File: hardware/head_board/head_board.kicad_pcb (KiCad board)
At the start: 2 copper layers, 90 x 74.7 mm, 121 parts, among them J1 8P8C, J2 CAM, J3 MOTOR, J4 MOTOR, J5 MOTOR, J6 CAMLED, SW1 BOOTSEL, U1 P78E05-1000, U2 MIC5317-3.3, U3 RP2040, U4 TVS, U5 W25Q128JVS, U6 TMC2209, U7 TMC2209, U8 TMC2209, U9 74HC2G34, Y1 12MHz

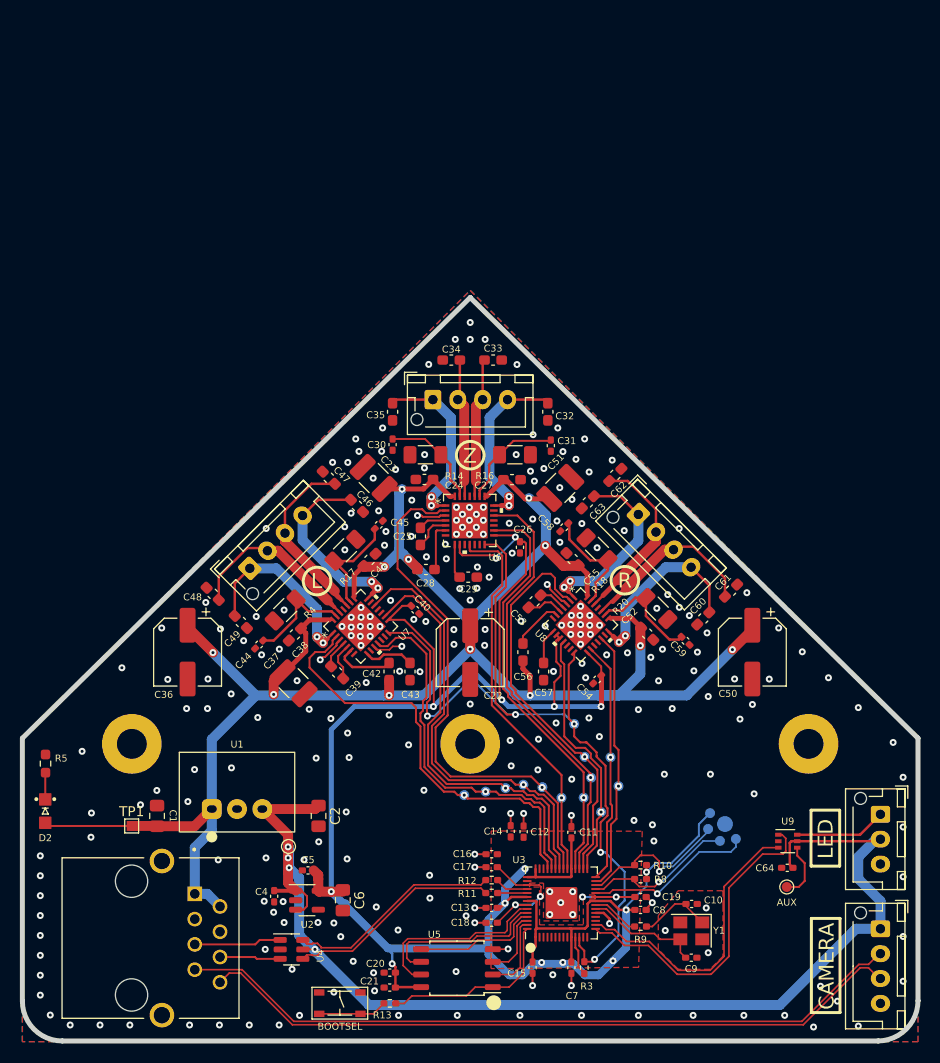
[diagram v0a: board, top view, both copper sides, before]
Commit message: Finish up layout for v1, ended up removing some stuff
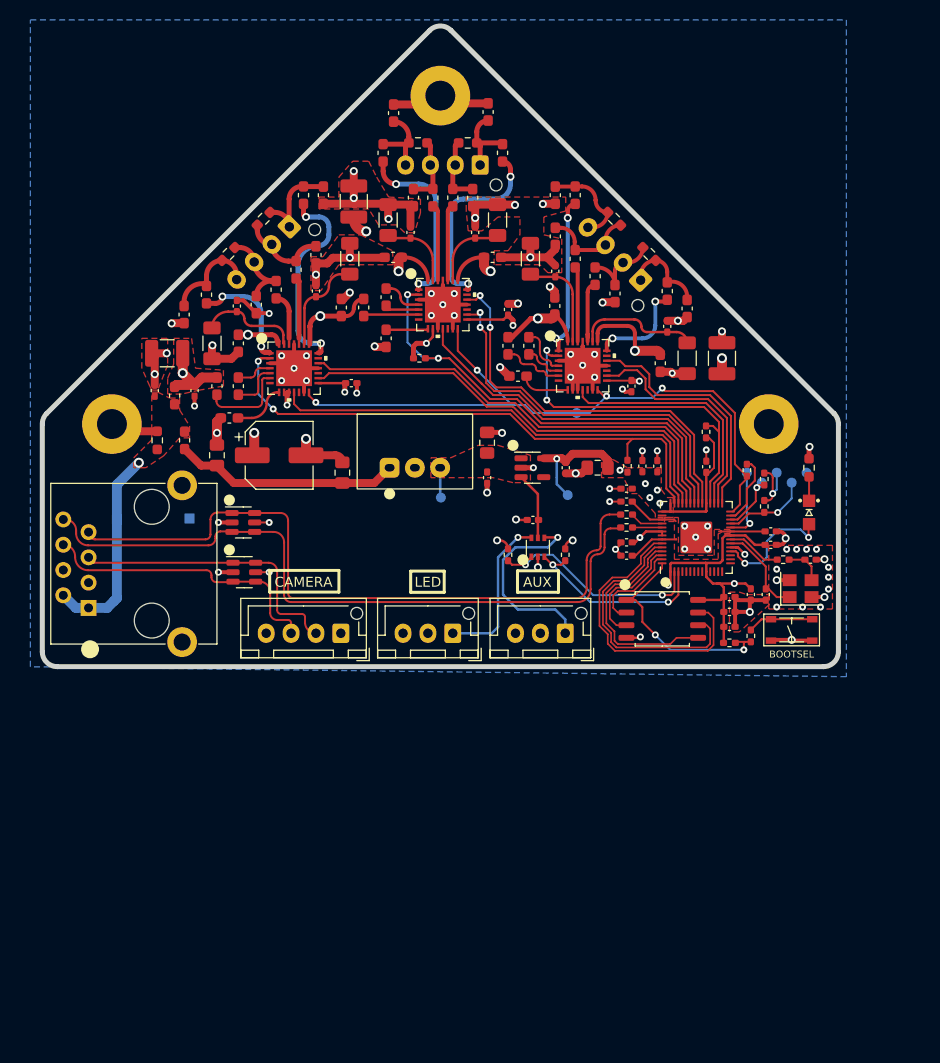
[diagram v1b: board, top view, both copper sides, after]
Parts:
- removed C1: 22u, Capacitor_SMD:C_0805_2012Metric_Pad1.18x1.45mm_HandSolder
- removed C22: 100u, Capacitor_SMD:CP_Elec_6.3x7.7
- removed the C25 at (103.2, 91.9)
- removed the C26 at (113.2, 93.0)
- removed the C28 at (103.8, 95.2)
- removed the C29 at (108.0, 96.0)
- removed the C36 at (79.8, 103.5)
- removed the C50 at (136.6, 103.5)
- removed the C64 at (140.1, 125.2)
- removed D2: 24V, winterbloom:LED_0805_Kingbright_APT2012
- removed G***: LOGO, winterbloom:Symbol_Winterbloom_40mm
- removed J1: 8P8C, winterbloom:Connector_RJ45_SS-7188S-A-PG4-BA-50
- removed J6: CAMLED, Connector_JST:JST_XH_B3B-XH-AM_1x03_P2.50mm_Vertical
- removed the R5 at (65.5, 114.7)
- removed TP10: M2STP, TestPoint:TestPoint_Pad_D1.0mm
- removed TP11: M2DAG, TestPoint:TestPoint_Pad_D1.0mm
- removed TP12: M2EN, TestPoint:TestPoint_Pad_D1.0mm
- removed TP13: M1DIR, TestPoint:TestPoint_Pad_D1.0mm
- removed TP14: M1STP, TestPoint:TestPoint_Pad_D1.0mm
- removed TP15: M1DAG, TestPoint:TestPoint_Pad_D1.0mm
- removed TP16: M1EN, TestPoint:TestPoint_Pad_D1.0mm
- removed TP18: M0STP, TestPoint:TestPoint_Pad_D1.0mm
- removed TP19: M0DAG, TestPoint:TestPoint_Pad_D1.0mm
- removed TP20: M0EN, TestPoint:TestPoint_Pad_D1.0mm
- removed TP21: UART, TestPoint:TestPoint_Pad_D1.0mm
- removed TP22: AUX, TestPoint:TestPoint_Pad_D1.0mm
- removed the U4 at (90.2, 133.4)
- removed the U9 at (140.1, 122.5)
- added C10: 10u, Capacitor_SMD:C_0805_2012Metric_Pad1.18x1.45mm_HandSolder, F.Cu at (121.0, 85.0)
- added C27: 100n, Capacitor_SMD:C_0402_1005Metric_Pad0.74x0.62mm_HandSolder, F.Cu at (114.5, 90.2)
- added C3: 22u, Capacitor_SMD:C_0805_2012Metric_Pad1.18x1.45mm_HandSolder, F.Cu at (82.8, 83.8)
- added C42: 22n, Capacitor_SMD:C_0603_1608Metric_Pad1.08x0.95mm_HandSolder, F.Cu at (99.8, 67.9)
- added C43: 100n, Capacitor_SMD:C_0402_1005Metric_Pad0.74x0.62mm_HandSolder, F.Cu at (112.0, 69.1)
- added C44: 100n, Capacitor_SMD:C_0603_1608Metric_Pad1.08x0.95mm_HandSolder, F.Cu at (97.5, 68.9)
- added C45: 4.7u, Capacitor_SMD:C_0603_1608Metric_Pad1.08x0.95mm_HandSolder, F.Cu at (99.8, 72.0)
- added C7: 1u, Capacitor_SMD:C_0402_1005Metric_Pad0.74x0.62mm_HandSolder, F.Cu at (117.8, 85.0)
- added C8: 100n, Capacitor_SMD:C_0402_1005Metric_Pad0.74x0.62mm_HandSolder, F.Cu at (76.5, 77.2)
- added C9: 100n, Capacitor_SMD:C_0402_1005Metric_Pad0.74x0.62mm_HandSolder, F.Cu at (80.5, 77.2)
- added D4: ACT, winterbloom:LED_0805_Kingbright_APT2012, F.Cu at (142.2, 89.5)
- added FB1: 50Ω @ 100MHz, Inductor_SMD:L_0603_1608Metric_Pad1.05x0.95mm_HandSolder, F.Cu at (78.5, 77.8)
- added FB10: 50Ω @ 100MHz, Inductor_SMD:L_0603_1608Metric_Pad1.05x0.95mm_HandSolder, F.Cu at (81.7, 67.6)
- added FB11: 50Ω @ 100MHz, Inductor_SMD:L_0603_1608Metric_Pad1.05x0.95mm_HandSolder, F.Cu at (88.7, 67.1)
- added FB12: 50Ω @ 100MHz, Inductor_SMD:L_0603_1608Metric_Pad1.05x0.95mm_HandSolder, F.Cu at (90.7, 65.1)
- added FB13: 50Ω @ 100MHz, Inductor_SMD:L_0603_1608Metric_Pad1.05x0.95mm_HandSolder, F.Cu at (91.5, 57.6)
- added FB14: 50Ω @ 100MHz, Inductor_SMD:L_0603_1608Metric_Pad1.05x0.95mm_HandSolder, F.Cu at (79.5, 82.2)
- added FB2: 50Ω @ 100MHz, Inductor_SMD:L_0603_1608Metric_Pad1.05x0.95mm_HandSolder, F.Cu at (118.8, 57.6)
- added FB3: 50Ω @ 100MHz, Inductor_SMD:L_0603_1608Metric_Pad1.05x0.95mm_HandSolder, F.Cu at (118.8, 64.0)
- added FB4: 50Ω @ 100MHz, Inductor_SMD:L_0603_1608Metric_Pad1.05x0.95mm_HandSolder, F.Cu at (120.8, 65.8)
- added FB5: 50Ω @ 100MHz, Inductor_SMD:L_0603_1608Metric_Pad1.05x0.95mm_HandSolder, F.Cu at (128.0, 67.2)
- added FB6: 50Ω @ 100MHz, Inductor_SMD:L_0603_1608Metric_Pad1.05x0.95mm_HandSolder, F.Cu at (99.5, 53.4)
- added FB7: 50Ω @ 100MHz, Inductor_SMD:L_0603_1608Metric_Pad1.05x0.95mm_HandSolder, F.Cu at (104.5, 57.9)
- added FB8: 50Ω @ 100MHz, Inductor_SMD:L_0603_1608Metric_Pad1.05x0.95mm_HandSolder, F.Cu at (106.5, 57.9)
- added FB9: 50Ω @ 100MHz, Inductor_SMD:L_0603_1608Metric_Pad1.05x0.95mm_HandSolder, F.Cu at (111.5, 53.4)
- added J3: CAM, Connector_JST:JST_XH_B4B-XH-AM_1x04_P2.50mm_Vertical, F.Cu at (95.2, 101.6)
- added J4: CAMLED, Connector_JST:JST_XH_B3B-XH-AM_1x03_P2.50mm_Vertical, F.Cu at (106.5, 101.6)
- added J5: AUX, Connector_JST:JST_XH_B3B-XH-AM_1x03_P2.50mm_Vertical, F.Cu at (117.8, 101.6)
- added R10: 1k, Resistor_SMD:R_0603_1608Metric_Pad0.98x0.95mm_HandSolder, F.Cu at (142.2, 85.0)
- added R12: 10k, Resistor_SMD:R_0402_1005Metric_Pad0.72x0.64mm_HandSolder, F.Cu at (134.2, 102.6)
- added R13: 10k, Resistor_SMD:R_0402_1005Metric_Pad0.72x0.64mm_HandSolder, F.Cu at (112.0, 93.8)
- added R14: 10k, Resistor_SMD:R_0402_1005Metric_Pad0.72x0.64mm_HandSolder, F.Cu at (117.8, 93.8)
- added R17: 10k, Resistor_SMD:R_0402_1005Metric_Pad0.72x0.64mm_HandSolder, F.Cu at (131.9, 81.4)
- added R20: 10k, Resistor_SMD:R_0402_1005Metric_Pad0.72x0.64mm_HandSolder, F.Cu at (103.1, 74.0)
- added R23: 10k, Resistor_SMD:R_0402_1005Metric_Pad0.72x0.64mm_HandSolder, F.Cu at (124.0, 84.8)
- added RV1: 35V, Resistor_SMD:R_0603_1608Metric_Pad0.98x0.95mm_HandSolder, F.Cu at (76.8, 82.2)
- added RV2: 35V, Resistor_SMD:R_0603_1608Metric_Pad0.98x0.95mm_HandSolder, F.Cu at (122.7, 60.0)
- added RV3: 35V, Resistor_SMD:R_0603_1608Metric_Pad0.98x0.95mm_HandSolder, F.Cu at (126.2, 63.5)
- added RV4: 35V, Resistor_SMD:R_0603_1608Metric_Pad0.98x0.95mm_HandSolder, F.Cu at (103.0, 52.4)
- added RV5: 35V, Resistor_SMD:R_0603_1608Metric_Pad0.98x0.95mm_HandSolder, F.Cu at (108.0, 52.4)
- added RV6: 35V, Resistor_SMD:R_0603_1608Metric_Pad0.98x0.95mm_HandSolder, F.Cu at (83.9, 63.5)
- added RV7: 35V, Resistor_SMD:R_0603_1608Metric_Pad0.98x0.95mm_HandSolder, F.Cu at (87.4, 60.0)
- added U5: TVS, Package_TO_SOT_SMD:SOT-23-6, F.Cu at (85.5, 95.5)
- added U6: TVS, Package_TO_SOT_SMD:SOT-23-6, F.Cu at (85.4, 90.5)
- added U7: 74HC2G34, Package_TO_SOT_SMD:SOT-363_SC-70-6, F.Cu at (115.0, 93.0)
- C2: value 22u -> 4.7u
- C4: value 1u -> 22u; footprint Capacitor_SMD:C_0402_1005Metric_Pad0.74x0.62mm_HandSolder -> Capacitor_SMD:C_0805_2012Metric_Pad1.18x1.45mm_HandSolder
- C5: value 1u -> 100u; footprint Capacitor_SMD:C_0402_1005Metric_Pad0.74x0.62mm_HandSolder -> Capacitor_SMD:CP_Elec_6.3x7.7
- C6: value 10u -> 1u; footprint Capacitor_SMD:C_0805_2012Metric_Pad1.18x1.45mm_HandSolder -> Capacitor_SMD:C_0402_1005Metric_Pad0.74x0.62mm_HandSolder
- J2: value CAM -> 8P8C; footprint Connector_JST:JST_XH_B4B-XH-AM_1x04_P2.50mm_Vertical -> winterbloom:Connector_RJ45_ASSMANN_A-2014-2S-4-N-R
- J7: renamed from J4; moved to B.Cu
- J8: renamed from J3; moved to B.Cu
- J9: renamed from J5; moved to B.Cu
- R11: renamed from R9; value 1K -> 1k
- R18: renamed from R4; value 22R -> 220m
- R19: renamed from R17; value 22R -> 220m
- R21: renamed from R14; value 22R -> 220m
- R22: renamed from R16; value 22R -> 220m
- R24: renamed from R18; value 22R -> 220m
- R25: renamed from R20; value 22R -> 220m
- R4: renamed from R10; value 10K -> 10k
- R5: renamed from R8; value 10K -> 10k
- R8: renamed from R3; value 1K -> 1k
- R9: renamed from R13; value 1K -> 1k
- TP1: value 24V -> GND; moved to B.Cu
- TP17: value M0DIR -> UART
- TP2: value 5V -> 24V; footprint TestPoint:TestPoint_Pad_D1.0mm -> TestPoint:TestPoint_Pad_1.0x1.0mm; moved to B.Cu
- TP3: value 3V3 -> 5V
- TP5: value RST -> GND
- TP6: value SWD -> 3V3
- TP7: value SWCLK -> ~{RST}
- TP8: value GND -> SWD
- TP9: value M2DIR -> SWC
- U1: value P78E05-1000 -> VX7805-500; footprint winterbloom:Converter_DCDC_CUI_P78E-1000_THT -> winterbloom:Converter_DCDC_CUI_VX78-500_THT
- moved J2 81.9 mm to (76.2, 94.6)
- moved H3 65.2 mm to (105.2, 47.6)
- moved SW1 58.9 mm to (140.5, 101.3), turned to 0 degrees
- moved C67 57.1 mm to (93.5, 57.6), turned to -90 degrees
- moved C35 54.0 mm to (133.5, 74.0), turned to 90 degrees
- moved C69 53.6 mm to (92.7, 63.6), turned to -90 degrees
- moved C40 53.3 mm to (116.8, 57.6), turned to -90 degrees
- moved R8 52.6 mm to (136.0, 85.2), turned to -90 degrees
- moved R9 51.8 mm to (136.4, 101.9), turned to -90 degrees
- moved C61 51.1 mm to (92.7, 67.2), turned to 90 degrees
- moved C4 50.4 mm to (109.9, 82.5), turned to 90 degrees
- moved C25 49.8 mm to (134.2, 101.0), turned to 0 degrees
- moved C26 49.8 mm to (134.2, 99.5), turned to 0 degrees
- moved C38 49.8 mm to (116.8, 61.8), turned to -90 degrees
- moved U2 49.0 mm to (114.5, 85.0)
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- renumbered C7 to C11, C8 to C12, C11 to C13, C12 to C14, C13 to C15, C14 to C16, C15 to C17, C16 to C18, C17 to C19, C18 to C20, C19 to C21, C9 to C23, C10 to C24, C21 to C25, C20 to C26, C39 to C28, C40 to C29, C42 to C30, C43 to C31, C44 to C32, C45 to C33, C37 to C35, C38 to C36, C41 to C37, C48 to C38, C46 to C39, C49 to C40, C47 to C41, C30 to C46, C31 to C47, C23 to C49, C24 to C50, C27 to C51, C34 to C52, C32 to C53, C35 to C54, C33 to C55, C53 to C56, C54 to C57, C56 to C58, C57 to C59, C58 to C60, C59 to C61, C51 to C63, C52 to C64, C55 to C65, C62 to C66, C60 to C67, C63 to C68, C61 to C69, R11 to R6, R12 to R7, U8 to U10, U5 to U4, U7 to U8, U6 to U9
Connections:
- net /MCU/QSPI_CS renamed /Microcontroller/QSPI_CS
- net /MCU/QSPI_SCLK renamed /Microcontroller/QSPI_SCLK
- net /MCU/QSPI_SD0 renamed /Microcontroller/QSPI_SD0
- net /MCU/QSPI_SD1 renamed /Microcontroller/QSPI_SD1
- net /MCU/QSPI_SD2 renamed /Microcontroller/QSPI_SD2
- net /MCU/QSPI_SD3 renamed /Microcontroller/QSPI_SD3
- net /MCU/XOUT renamed /Microcontroller/XOUT
- C2 pad 1: +5V -> Net-(C2-Pad1)
- C23 pad 1: /MCU/XIN -> /Microcontroller/XIN
- C24 pad 1: Net-(C10-Pad1) -> Net-(C24-Pad1)
- C30 pad 1: +24V -> VMOTOR
- C35 pad 1: +24V -> VMOTOR
- C36 pad 1: +24V -> VMOTOR
- C37 pad 1: +24V -> VMOTOR
- C38 pad 1: Net-(C48-Pad1) -> Net-(C38-Pad1)
- C39 pad 1: Net-(C46-Pad1) (its old number) -> Net-(C39-Pad1)
- C40 pad 1: Net-(C49-Pad1) -> Net-(C40-Pad1)
- C41 pad 1: Net-(C47-Pad1) (its old number) -> Net-(C41-Pad1)
- C49 pad 1: +24V -> VMOTOR
- C5 pad 1: +3V3 -> VMOTOR
- C50 pad 1: +24V -> VMOTOR
- C51 pad 1: +24V -> VMOTOR
- C52 pad 1: Net-(C34-Pad1) -> Net-(C52-Pad1)
- C53 pad 1: Net-(C32-Pad1) (its old number) -> Net-(C53-Pad1)
- C54 pad 1: Net-(C35-Pad1) -> Net-(C54-Pad1)
- C55 pad 1: Net-(C33-Pad1) (its old number) -> Net-(C55-Pad1)
- C58 pad 1: +24V -> VMOTOR
- C6 pad 1: +3V3 -> +5V
- C63 pad 1: +24V -> VMOTOR
- C64 pad 1: +24V -> VMOTOR
- C65 pad 1: +24V -> VMOTOR
- C66 pad 1: Net-(C62-Pad1) -> Net-(C66-Pad1)
- C67 pad 1: Net-(C60-Pad1) (its old number) -> Net-(C67-Pad1)
- C68 pad 1: Net-(C63-Pad1) -> Net-(C68-Pad1)
- C69 pad 1: Net-(C61-Pad1) (its old number) -> Net-(C69-Pad1)
- J2 pad 1: +5V -> +24V
- J2 pad 2: /Connections/CAM_D- -> +24V
- J2 pad 3: /Connections/CAM_D+ -> GND
- J7 pad 1: Net-(C49-Pad1) -> Net-(C39-Pad1)
- J7 pad 2: Net-(C48-Pad1) -> Net-(C41-Pad1)
- J7 pad 3: Net-(C47-Pad1) (its old number) -> Net-(C38-Pad1)
- J7 pad 4: Net-(C46-Pad1) (its old number) -> Net-(C40-Pad1)
- J8 pad 1: Net-(C35-Pad1) -> Net-(C53-Pad1)
- J8 pad 2: Net-(C34-Pad1) -> Net-(C55-Pad1)
- J8 pad 3: Net-(C33-Pad1) (its old number) -> Net-(C52-Pad1)
- J8 pad 4: Net-(C32-Pad1) (its old number) -> Net-(C54-Pad1)
- J9 pad 1: Net-(C63-Pad1) -> Net-(C67-Pad1)
- J9 pad 2: Net-(C62-Pad1) -> Net-(C69-Pad1)
- J9 pad 3: Net-(C61-Pad1) (its old number) -> Net-(C66-Pad1)
- J9 pad 4: Net-(C60-Pad1) (its old number) -> Net-(C68-Pad1)
- R11 pad 2: Net-(C10-Pad1) -> Net-(C24-Pad1)
- R4 pad 1: /MCU/RUN -> /Microcontroller/RUN
- R5 pad 2: /MCU/SWD -> /Microcontroller/SWD
- R6 pad 1: /MCU/USB_D+ -> /Microcontroller/USB_D+
- R7 pad 1: /MCU/USB_D- -> /Microcontroller/USB_D-
- R8 pad 1: /MCU/UART1_TX -> /Microcontroller/UART1_TX
- TP1 pad 1: +24V -> GND
- TP17 pad 1: /Left Motor/DIR -> /TMC_UART
- TP2 pad 1: +5V -> +24V
- TP3 pad 1: +3V3 -> +5V
- TP5 pad 1: /MCU/RUN -> GND
- TP6 pad 1: /MCU/SWD -> +3V3
- TP7 pad 1: /MCU/SWCLK -> /Microcontroller/RUN
- TP8 pad 1: GND -> /Microcontroller/SWD
- TP9 pad 1: /MCU/M2_DIR -> /Microcontroller/SWCLK
- U1 pad 1: +24V -> Net-(C2-Pad1)
- U10 pad 1: Net-(C63-Pad1) -> /Right Motor/OB2
- U10 pad 11: /MCU/M2_DIAG -> /Microcontroller/M2_DIAG
- U10 pad 16: /MCU/M2_STEP -> /Microcontroller/M2_STEP
- U10 pad 19: /MCU/M2_DIR -> /Microcontroller/M2_DIR
- U10 pad 2: /MCU/M2_EN -> /Microcontroller/M2_EN
- U10 pad 21: Net-(C60-Pad1) (its old number) -> /Right Motor/OA2
- U10 pad 22: +24V -> VMOTOR
- U10 pad 24: Net-(C61-Pad1) (its old number) -> /Right Motor/OA1
- U10 pad 26: Net-(C62-Pad1) -> /Right Motor/OB1
- U10 pad 28: +24V -> VMOTOR
- U3 pad 11: /MCU/UART1_TX -> unconnected-(U3-Pad11)
- U3 pad 12: /TMC_UART -> unconnected-(U3-Pad12)
- U3 pad 15: /MCU/CAM_LED_LV -> unconnected-(U3-Pad15)
- U3 pad 16: /MCU/AUX_LV -> unconnected-(U3-Pad16)
- U3 pad 18: unconnected-(U3-Pad18) -> /Microcontroller/ACT_LED
- U3 pad 2: unconnected-(U3-Pad2) -> /Connections/CAM_LED
- U3 pad 20: /MCU/XIN -> /Microcontroller/XIN
- U3 pad 24: /MCU/SWCLK -> /Microcontroller/SWCLK
- U3 pad 25: /MCU/SWD -> /Microcontroller/SWD
- U3 pad 26: /MCU/RUN -> /Microcontroller/RUN
- U3 pad 27: /MCU/M2_DIR -> /Microcontroller/UART1_TX
- U3 pad 28: /MCU/M2_STEP -> /TMC_UART
- U3 pad 29: /MCU/M2_DIAG -> /Left Motor/DIR
- U3 pad 3: unconnected-(U3-Pad3) -> /Connections/AUX_OUT
- U3 pad 30: /MCU/M2_EN -> /Left Motor/STEP
- U3 pad 31: /MCU/M1_DIR -> /Left Motor/DIAG
- U3 pad 32: /MCU/M1_STEP -> /Left Motor/ENN
- U3 pad 34: /MCU/M1_DIAG -> /Microcontroller/M1_DIR
- U3 pad 35: /MCU/M1_EN -> /Microcontroller/M1_STEP
- U3 pad 36: /Left Motor/DIR -> /Microcontroller/M1_DIAG
- U3 pad 37: /Left Motor/STEP -> /Microcontroller/M1_EN
- U3 pad 38: /Left Motor/DIAG -> /Microcontroller/M2_DIR
- U3 pad 39: /Left Motor/ENN -> /Microcontroller/M2_STEP
- U3 pad 40: unconnected-(U3-Pad40) -> /Microcontroller/M2_DIAG
- U3 pad 41: unconnected-(U3-Pad41) -> /Microcontroller/M2_EN
- U8 pad 1: Net-(C49-Pad1) -> /Left Motor/OB2
- U8 pad 21: Net-(C46-Pad1) (its old number) -> /Left Motor/OA2
- U8 pad 22: +24V -> VMOTOR
- U8 pad 24: Net-(C47-Pad1) (its old number) -> /Left Motor/OA1
- U8 pad 26: Net-(C48-Pad1) -> /Left Motor/OB1
- U8 pad 28: +24V -> VMOTOR
- U9 pad 1: Net-(C35-Pad1) -> /Z Motor/OB2
- U9 pad 11: /MCU/M1_DIAG -> /Microcontroller/M1_DIAG
- U9 pad 16: /MCU/M1_STEP -> /Microcontroller/M1_STEP
- U9 pad 19: /MCU/M1_DIR -> /Microcontroller/M1_DIR
- U9 pad 2: /MCU/M1_EN -> /Microcontroller/M1_EN
- U9 pad 21: Net-(C32-Pad1) (its old number) -> /Z Motor/OA2
- U9 pad 22: +24V -> VMOTOR
- U9 pad 24: Net-(C33-Pad1) (its old number) -> /Z Motor/OA1
- U9 pad 26: Net-(C34-Pad1) -> /Z Motor/OB1
- U9 pad 28: +24V -> VMOTOR
- Y1 pad 1: Net-(C10-Pad1) -> /Microcontroller/XIN
- Y1 pad 3: /MCU/XIN -> Net-(C24-Pad1)
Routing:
- net +24V: track 211.3 -> 20.8 mm, vias 12 -> 1
- net GND: track 27.8 -> 168.6 mm, vias 266 -> 84
- net VMOTOR: track 0.00 -> 137.4 mm, vias 0 -> 10
- net /Microcontroller/USB_D-: track 0.00 -> 70.7 mm
- net /Microcontroller/USB_D+: track 0.00 -> 70.1 mm
- net /Microcontroller/M2_EN: track 0.00 -> 56.4 mm, vias 0 -> 2
- net /MCU/M1_EN: track 53.1 -> 0.00 mm, vias 1 -> 0
- net +5V: track 118.8 -> 71.0 mm, vias 4 -> 2
- net /Microcontroller/M2_DIAG: track 0.00 -> 47.0 mm
- net /Microcontroller/M2_DIR: track 0.00 -> 46.1 mm
- net /Microcontroller/M1_EN: track 0.00 -> 45.7 mm, vias 0 -> 2
- net /Microcontroller/M2_STEP: track 0.00 -> 45.4 mm
- net /Connections/CAM_D-: track 73.8 -> 29.0 mm
- net /MCU/M1_DIR: track 43.6 -> 0.00 mm, vias 1 -> 0
- net /Connections/CAM_D+: track 71.6 -> 28.8 mm
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- added copper zone on F.Cu, net +24V
- added copper zone on In2.Cu, net +3V3
- added copper zone on F.Cu, net +5V
- added copper zone on In1.Cu, net GND
- added copper zone on F.Cu, net VMOTOR
- added copper zone on In2.Cu, net VMOTOR
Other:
- board size 90 x 74.7 mm -> 80 x 64.4 mm
- copper layers 2 -> 4
- board text added: "${TITLE} ${REVISION} ${ISSUE_DATE} ${COMPANY} ${COMMENT3} ${COMMENT2} ${COMMENT1}"
- board text added: "AUX"
- board text removed: "${TITLE} ${REVISION} ${ISSUE_DATE} ${COMMENT1} ${COMMENT2} ${COMMENT3}"
- board text removed: "L"
- board text removed: "R"
- board text removed: "TRANS RIGHTS"
- board text removed: "Z"
